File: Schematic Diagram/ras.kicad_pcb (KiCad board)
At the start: 2 copper layers, 18 parts, among them SW1 SHUTDOWN, SW2 HOME, SW3 MENU, SW4 PREVIOUS, SW5 RotaryEncoder_Switch, SW6 NEXT, SW7 DONE

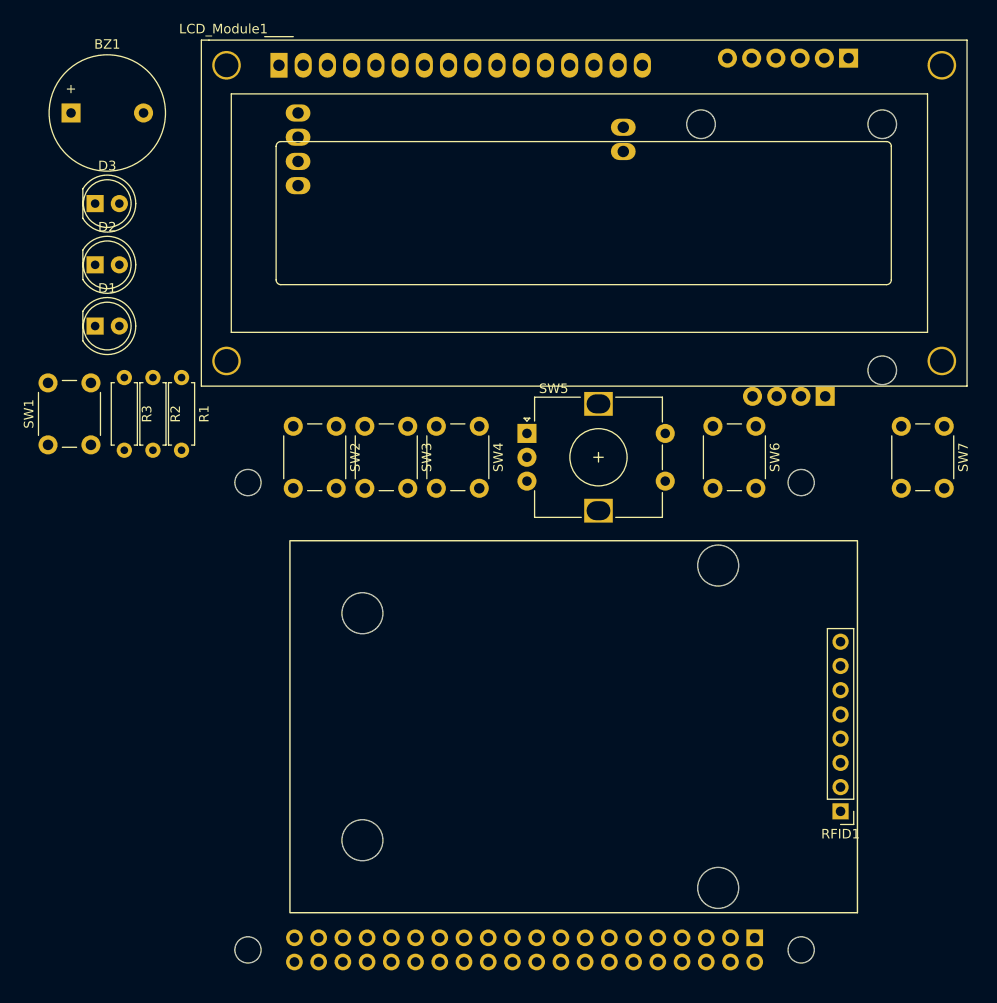
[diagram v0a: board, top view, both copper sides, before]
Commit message: wiring
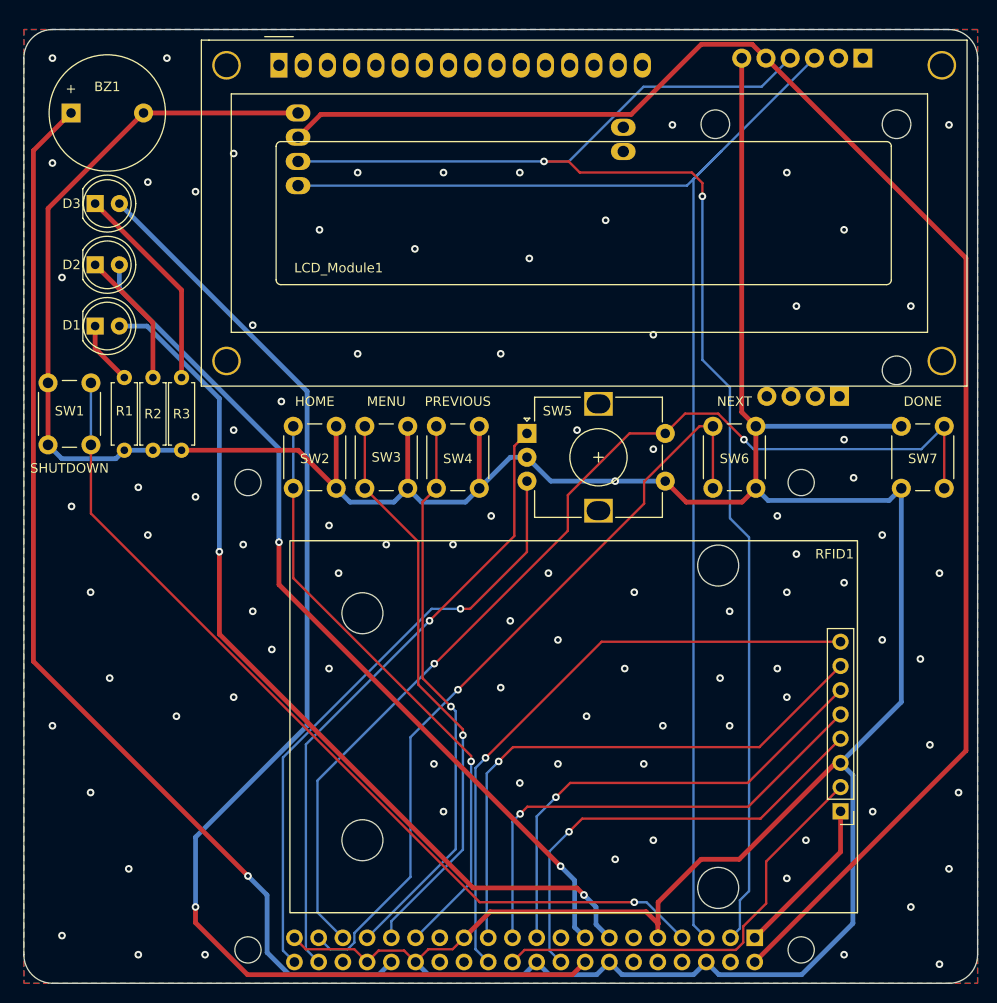
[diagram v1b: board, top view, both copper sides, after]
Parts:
- moved R1 9.70 mm to (164.8, 67.7), turned to 90 degrees
- moved R3 9.70 mm to (170.8, 67.7), turned to 90 degrees
- moved R2 7.62 mm to (167.8, 67.7), turned to 90 degrees
- moved U1 1.50 mm to (225.3, 25.3)
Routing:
- net GND: track 0.00 -> 408.0 mm, vias 0 -> 89
- net +5V: track 0.00 -> 166.3 mm
- net I2C_SDA: track 0.00 -> 155.6 mm, vias 0 -> 2
- net I2C_SCL: track 0.00 -> 143.9 mm
- net LED-BLUE: track 0.00 -> 132.1 mm, vias 0 -> 1
- net Buzzer: track 0.00 -> 119.6 mm, vias 0 -> 1
- net DONE_BUTTON: track 0.00 -> 110.5 mm, vias 0 -> 2
- net SHUTDOWN_BUTTON: track 0.00 -> 94.1 mm, vias 0 -> 1
- net LED-RED: track 0.00 -> 93.5 mm, vias 0 -> 2
- net LED-GREEN: track 0.00 -> 90.8 mm, vias 0 -> 2
- net NEXT_BUTTON: track 0.00 -> 81.6 mm, vias 0 -> 1
- net ENCODER_A: track 0.00 -> 65.6 mm, vias 0 -> 1
- net SPI_CE-RFID: track 0.00 -> 64.7 mm, vias 0 -> 1
- net HOME_BUTTON: track 0.00 -> 63.9 mm, vias 0 -> 1
- net ENCODER_B: track 0.00 -> 63.9 mm, vias 0 -> 1
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- added copper zone on B.Cu, net GND
- added copper zone on F.Cu, net GND
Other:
- board outline added: 100 x 100 mm
- board text added: "PCB Designed by souchan.jp"
